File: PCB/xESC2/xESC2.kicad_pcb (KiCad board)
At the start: 2 copper layers, 32.9 x 34.4 mm, 24 parts, among them Q1 BSC026N08NS5, Q2 BSC026N08NS5, Q3 BSC026N08NS5, Q4 BSC026N08NS5, Q5 BSC026N08NS5, Q6 BSC026N08NS5

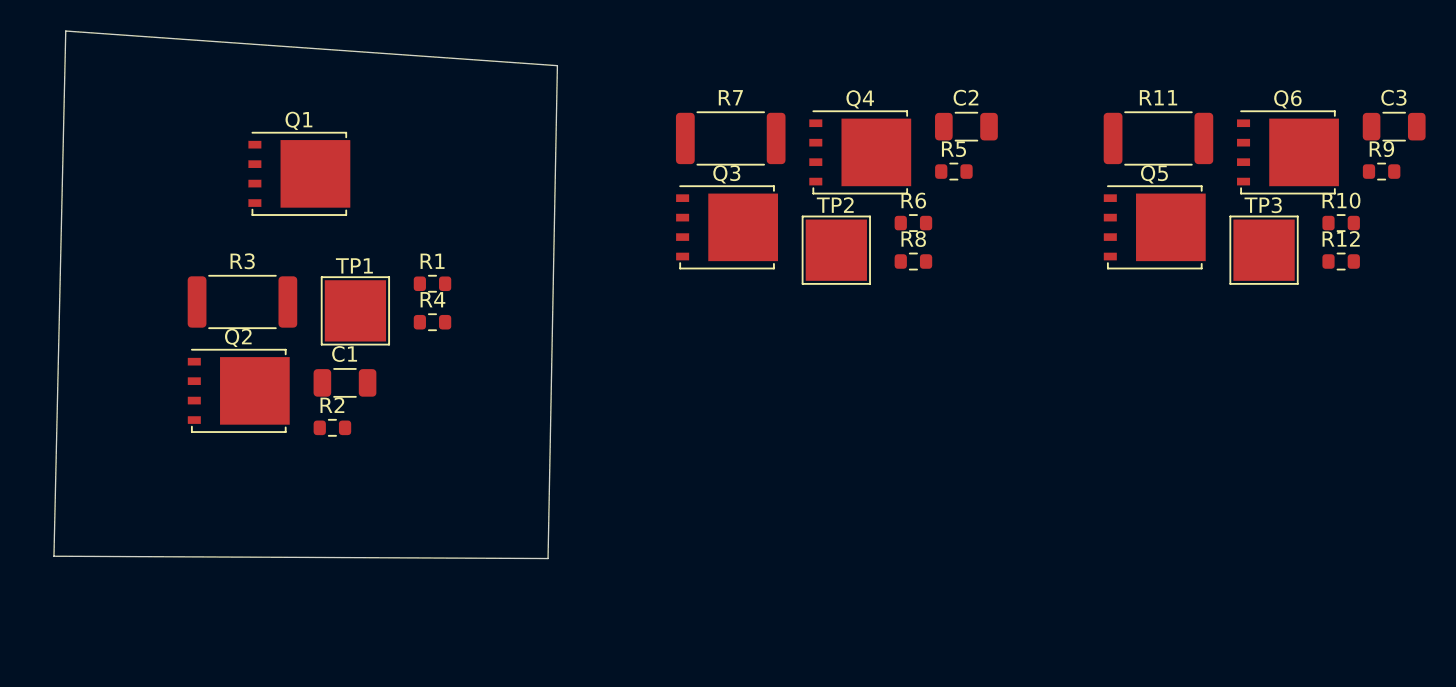
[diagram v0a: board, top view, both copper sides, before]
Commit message: power schematic wip
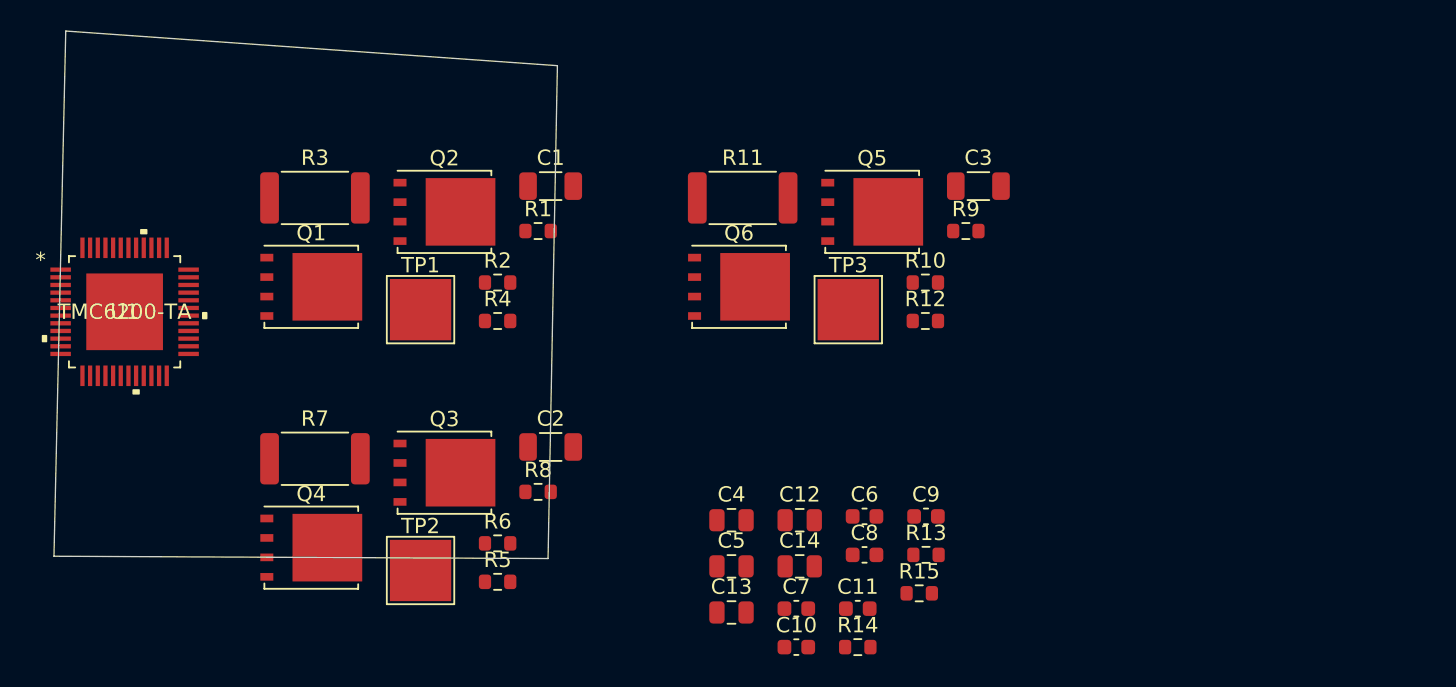
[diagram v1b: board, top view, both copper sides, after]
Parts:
- added C10: 470nF/16V, Capacitor_SMD:C_0603_1608Metric, F.Cu at (139.6, 105.1)
- added C11: 22nF/100V, Capacitor_SMD:C_0603_1608Metric, F.Cu at (143.6, 102.6)
- added C12: 100nF/100V, Capacitor_SMD:C_0805_2012Metric, F.Cu at (139.8, 96.8)
- added C13: 100nF/100V, Capacitor_SMD:C_0805_2012Metric, F.Cu at (135.4, 102.8)
- added C14: 100nF/100V, Capacitor_SMD:C_0805_2012Metric, F.Cu at (139.8, 99.8)
- added C4: 2.2uF/50V, Capacitor_SMD:C_0805_2012Metric, F.Cu at (135.4, 96.8)
- added C5: 2.2uF/50V, Capacitor_SMD:C_0805_2012Metric, F.Cu at (135.4, 99.8)
- added C6: 100nF/50V, Capacitor_SMD:C_0603_1608Metric, F.Cu at (144.1, 96.5)
- added C7: 100nF/50V, Capacitor_SMD:C_0603_1608Metric, F.Cu at (139.6, 102.6)
- added C8: 470nF/16V, Capacitor_SMD:C_0603_1608Metric, F.Cu at (144.1, 99.1)
- added C9: 470nF/16V, Capacitor_SMD:C_0603_1608Metric, F.Cu at (148.1, 96.5)
- added R13: DNP, Resistor_SMD:R_0603_1608Metric, F.Cu at (148.1, 99.1)
- added R14: DNP, Resistor_SMD:R_0603_1608Metric, F.Cu at (143.6, 105.1)
- added R15: DNP, Resistor_SMD:R_0603_1608Metric, F.Cu at (147.7, 101.6)
- added U1: TMC6200-TA, footprints:TMC6200-TA, F.Cu at (95.8, 83.2)
- moved Q4 44.1 mm to (108.0, 98.6)
- moved R5 40.0 mm to (120.1, 100.8)
- moved Q6 36.9 mm to (135.9, 81.6)
- moved R6 34.2 mm to (120.1, 98.3)
- moved R7 34.2 mm to (108.2, 92.8)
- moved TP2 34.2 mm to (115.1, 100.1)
- moved C2 34.2 mm to (123.6, 92.0)
- moved R8 28.7 mm to (122.8, 95.0)
- moved R10 27.4 mm to (148.1, 81.3)
- moved R9 27.4 mm to (150.7, 77.9)
- moved C3 27.4 mm to (151.5, 75.0)
- moved R11 27.4 mm to (136.1, 75.8)
- moved R12 27.4 mm to (148.1, 83.8)
- moved TP3 27.4 mm to (143.0, 83.1)
- moved Q3 24.4 mm to (116.7, 93.7)
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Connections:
- net /Power/MOSFET/DRV renamed /Power/DRV_U
- net /Power/sheet61A57DC9/DRV renamed /Power/DRV_V
- net /Power/sheet61A580CB/DRV renamed /Power/DRV_W
- C1 pad 1: /Power/MOSFET/VM -> /Power/VM
- C2 pad 1: /Power/sheet61A57DC9/VM -> /Power/VM
- C3 pad 1: /Power/sheet61A580CB/VM -> /Power/VM
- Q1 pad 5: /Power/MOSFET/VM -> /Power/VM
- Q3 pad 5: /Power/sheet61A57DC9/VM -> /Power/VM
- Q5 pad 5: /Power/sheet61A580CB/VM -> /Power/VM
- R1 pad 2: (no net) -> /Power/HSU
- R10 pad 2: (no net) -> /Power/LSW
- R12 pad 2: (no net) -> /Power/SENSE_W
- R2 pad 2: (no net) -> /Power/LSU
- R4 pad 2: (no net) -> /Power/SENSE_U
- R5 pad 2: (no net) -> /Power/HSV
- R6 pad 2: (no net) -> /Power/LSV
- R8 pad 2: (no net) -> /Power/SENSE_V
- R9 pad 2: (no net) -> /Power/HSW
